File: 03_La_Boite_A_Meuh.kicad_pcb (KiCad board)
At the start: 2 copper layers, 100 x 100 mm, 64 parts, among them J1 Micro_SD_Card, J10 Conn_01x01, J11 Conn_01x04, J18 Conn_01x02, J2 Conn_01x06, J26 Conn_01x02, J29 Conn_01x02, J3 Conn_01x08, J4 Conn_01x02, J5 Conn_02x02_Counter_Clockwise, J6 Conn_01x04, J7 Conn_01x04, J8 Conn_01x04, J9 USB_B_Micro, Q1 2N7002, U1 Audio_Facile, U2 ESP32-DEVKITC, U3 rot_pot_rot_sw, U4 Batt_Alim, U5 UDA1334_ADAFRUIT

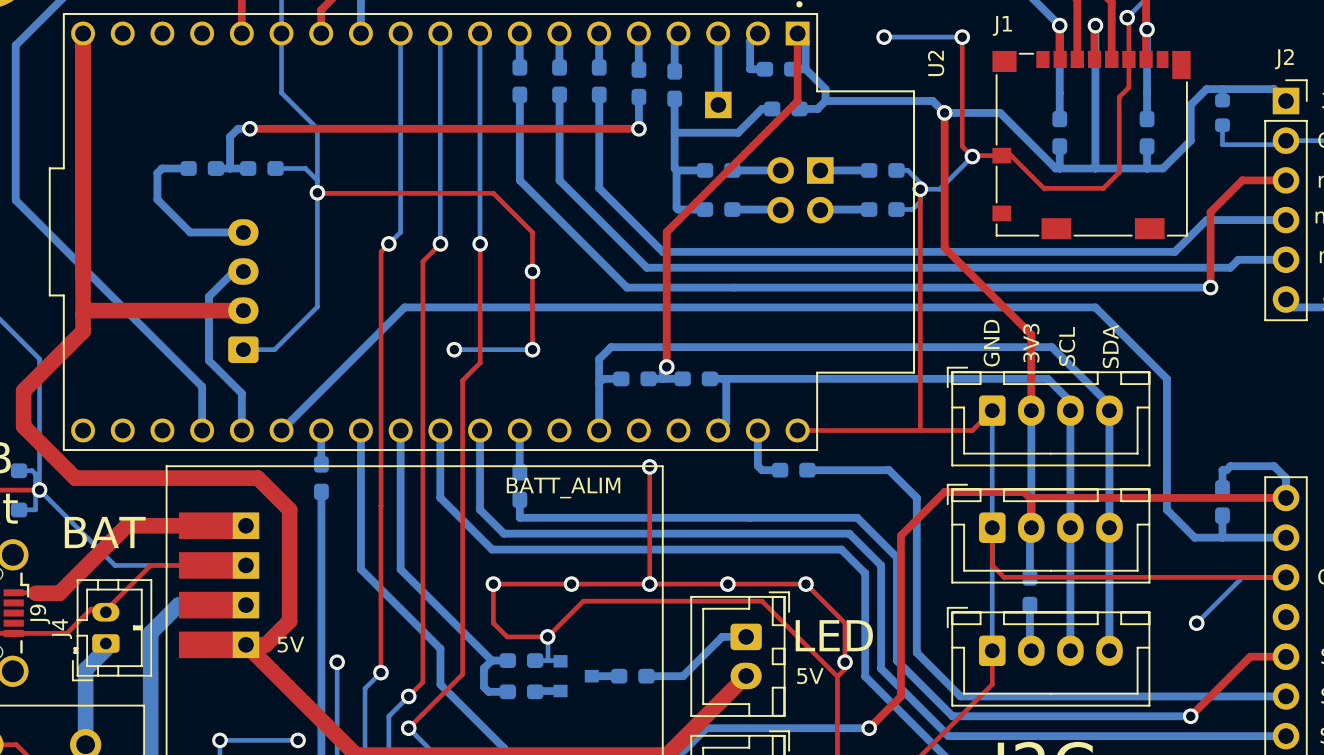
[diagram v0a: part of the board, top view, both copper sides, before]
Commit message: maj split librairie
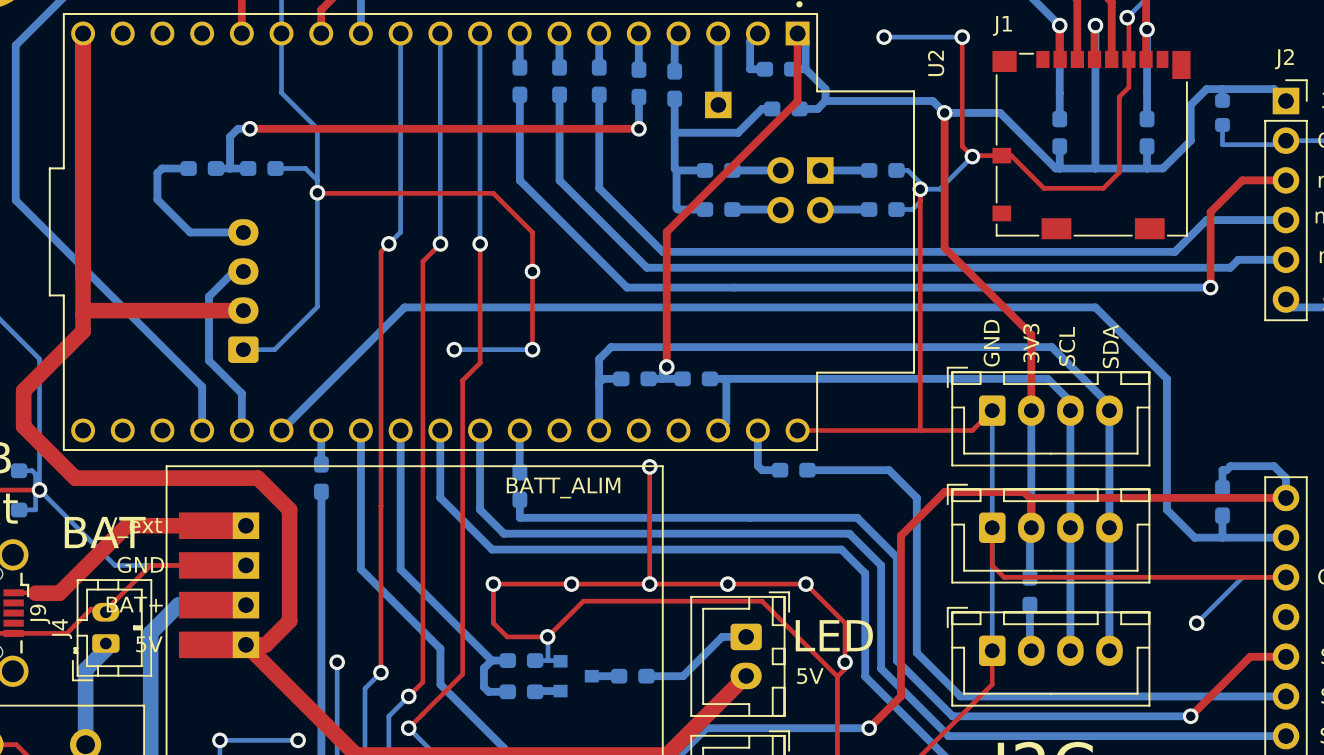
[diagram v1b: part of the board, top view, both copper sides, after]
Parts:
- U1: footprint Chimere:Audio_Facile -> Chimere_mods:Audio_Facile
- U2: footprint Chimere:MODULE_ESP32-DEVKITC -> Chimere_comps:MODULE_ESP32-DEVKITC
- U3: footprint Chimere:PTR901 -> Chimere_comps:PTR901
- U4: footprint Chimere:Batt_Alim -> Chimere_mods:Batt_Alim
- U5: footprint Chimere:Adafruit_UDA1334 -> Chimere_comps:Adafruit_UDA1334

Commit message: passage à la version "HP" de audio facile
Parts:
- U1: footprint Chimere_mods:Audio_Facile -> Chimere_mods:Audio_Facile_HP
